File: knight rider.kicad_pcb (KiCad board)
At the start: 2 copper layers, 65 x 85 mm, 28 parts, among them U1 ICM7555xB, U2 4017

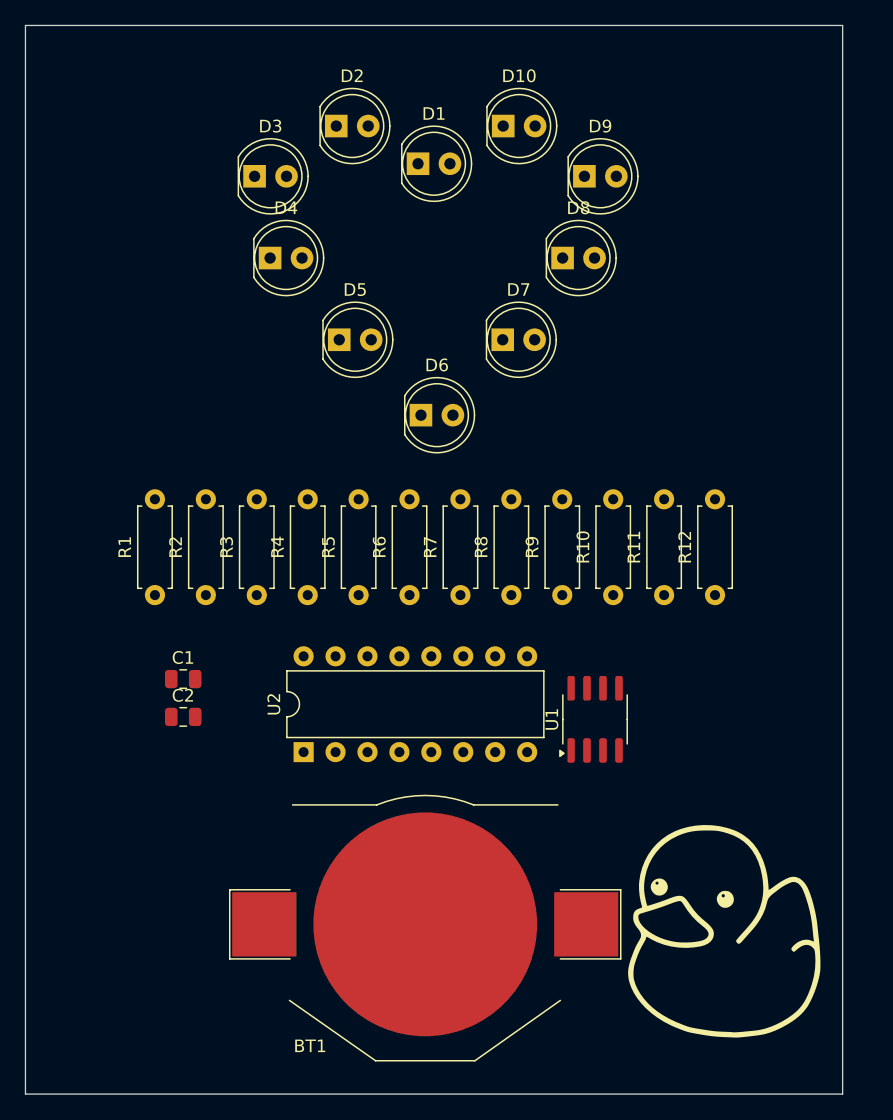
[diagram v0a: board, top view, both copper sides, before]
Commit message: Add files via upload
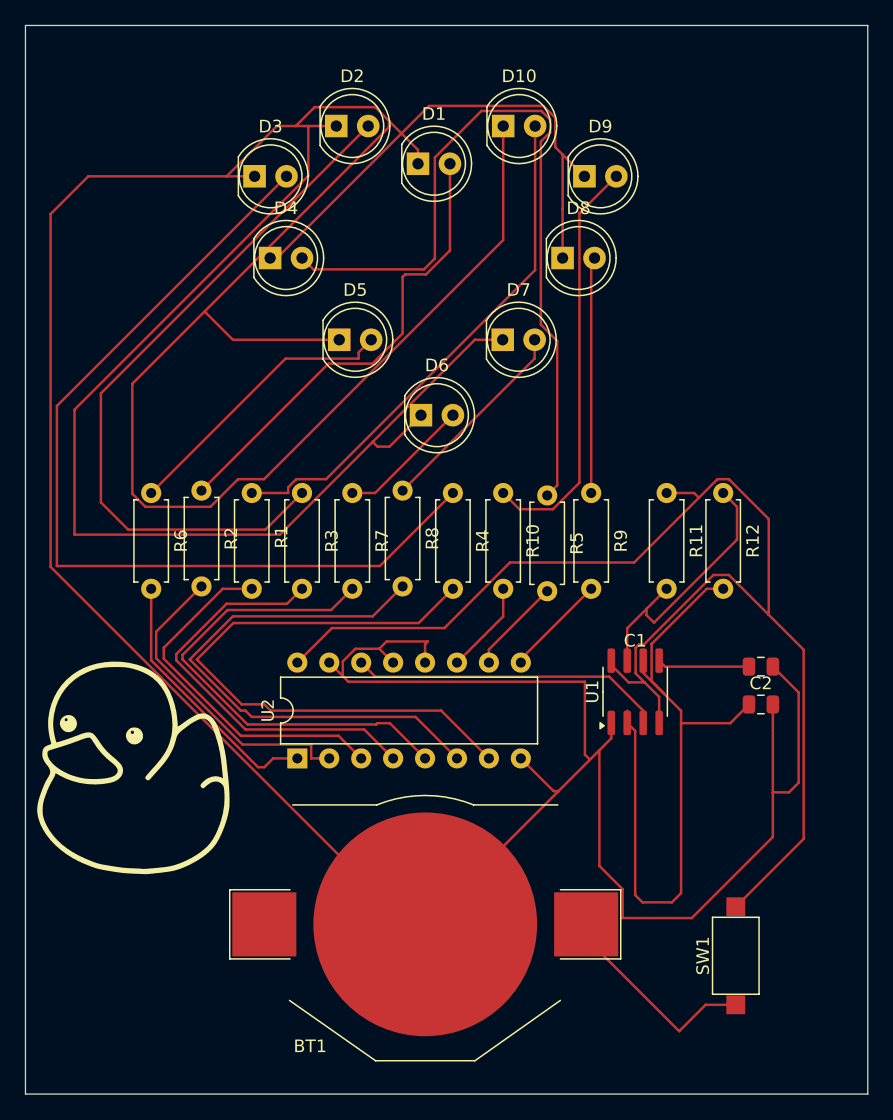
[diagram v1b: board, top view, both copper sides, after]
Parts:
- added SW1: SW_Push, Button_Switch_SMD:SW_SPST_CK_RS282G05A3, F.Cu at (157.0, 121.0)
- moved   48.8 mm to (109.0, 106.0)
- moved C1 46.0 mm to (159.0, 98.0)
- moved C2 46.0 mm to (159.0, 101.0)
- moved R6 22.1 mm to (110.5, 84.2), turned to -90 degrees
- moved R5 17.0 mm to (142.0, 84.4), turned to -90 degrees
- moved R4 14.1 mm to (134.5, 84.2), turned to -90 degrees
- moved R8 12.0 mm to (130.5, 84.0), turned to -90 degrees
- moved R10 11.9 mm to (138.5, 84.2), turned to -90 degrees
- moved R7 11.8 mm to (126.5, 84.2), turned to -90 degrees
- moved R1 11.2 mm to (118.5, 84.2), turned to -90 degrees
- moved R3 8.88 mm to (122.5, 84.2), turned to -90 degrees
- moved R9 8.44 mm to (145.5, 84.2), turned to -90 degrees
- moved R2 8.32 mm to (114.5, 84.0), turned to -90 degrees
- moved R12 8.15 mm to (156.0, 84.2), turned to -90 degrees
- moved R11 8.12 mm to (151.5, 84.2), turned to -90 degrees
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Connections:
- R11 pad 1: Net-(BT1-+) -> Net-(U1-R)
- U1 pad 4: Net-(BT1-+) -> Net-(U1-R)
- U1 pad 8: Net-(BT1-+) -> Net-(U1-R)
- U2 pad 12: unconnected-(U2-Cout-Pad12) -> Net-(BT1--)
- U2 pad 16: Net-(BT1-+) -> Net-(U1-R)
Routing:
- net Net-(BT1--): track 0.00 -> 458.4 mm
- net Net-(U1-R): track 0.00 -> 106.4 mm
- net Net-(D3-A): track 0.00 -> 72.5 mm
- net Net-(D4-A): track 0.00 -> 61.4 mm
- net Net-(D2-A): track 0.00 -> 56.8 mm
- net Net-(U1-THR): track 0.00 -> 56.8 mm
- net Net-(U2-Q3): track 0.00 -> 49.2 mm
- net Net-(U2-Q7): track 0.00 -> 43.9 mm
- net Net-(D10-A): track 0.00 -> 41.6 mm
- net Net-(U2-Q6): track 0.00 -> 38.7 mm
- net Net-(D1-A): track 0.00 -> 37.2 mm
- net Net-(U2-Q2): track 0.00 -> 33.1 mm
- net Net-(D9-A): track 0.00 -> 33.1 mm
- net Net-(U2-Q0): track 0.00 -> 28.8 mm
- net Net-(U1-Q): track 0.00 -> 25.0 mm
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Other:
- board size 65 x 85 mm -> 67 x 85 mm
